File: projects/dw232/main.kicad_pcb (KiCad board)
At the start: 4 copper layers, 99 x 25 mm, 27 parts, among them P101 CONN_01X07, Q501 MMBT3904, Q502 MMBT3904, U501 LM741, U502 LM741, U503 2DW232

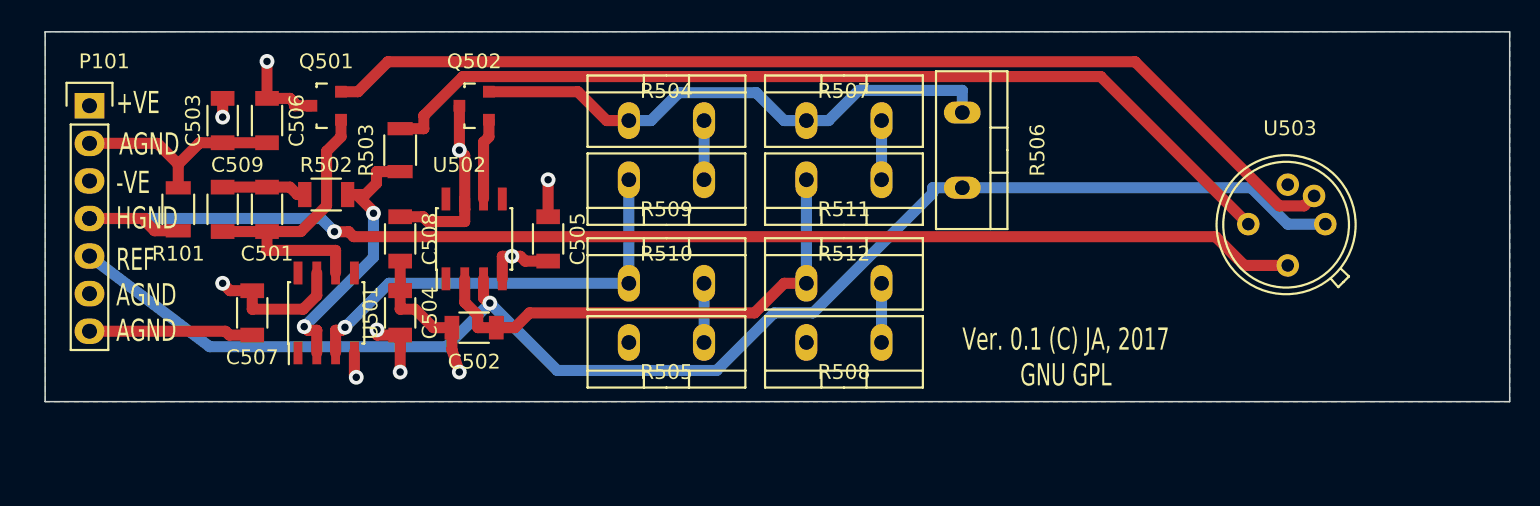
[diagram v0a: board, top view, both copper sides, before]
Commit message: adjust positions
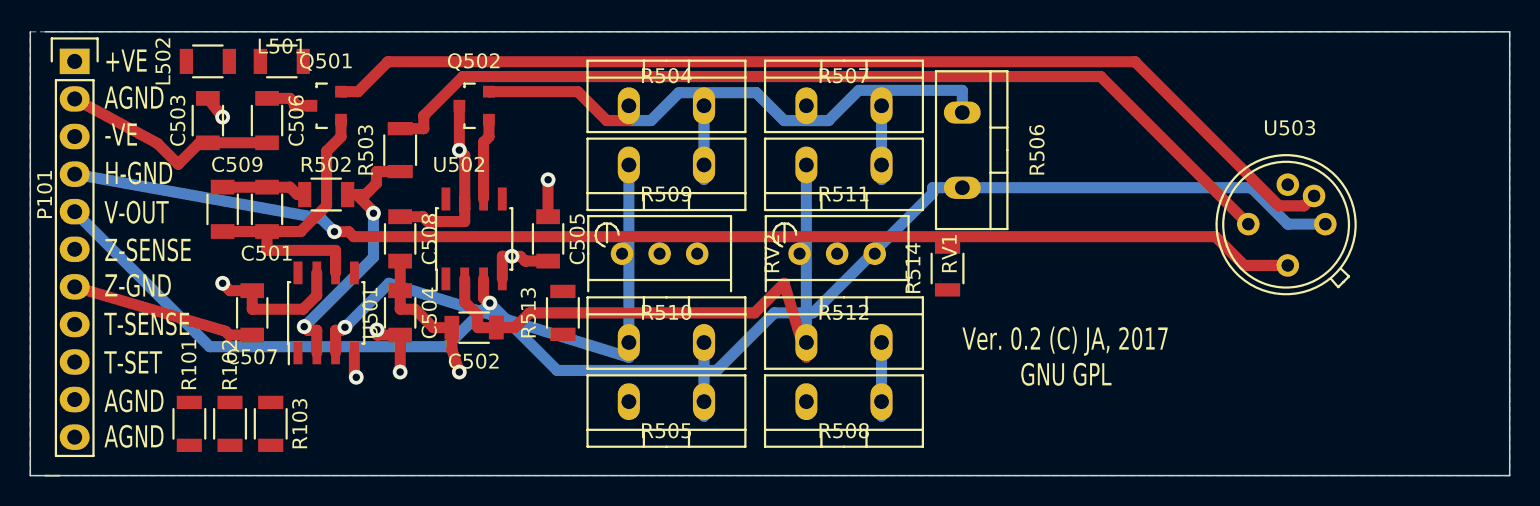
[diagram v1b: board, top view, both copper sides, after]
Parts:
- added L501: INDUCTOR, Resistors_SMD:R_1206, F.Cu at (56.0, 31.0)
- added L502: INDUCTOR, Resistors_SMD:R_1206, F.Cu at (51.0, 31.0)
- added R102: 0R, Resistors_SMD:R_1206, F.Cu at (52.5, 55.5)
- added R103: 0R, Resistors_SMD:R_1206, F.Cu at (55.2, 55.5)
- added R513: 0R, Resistors_SMD:R_1206, F.Cu at (75.0, 48.0)
- added R514: 0R, Resistors_SMD:R_1206, F.Cu at (101.0, 45.0)
- added RV1: 1k, Potentiometers:Potentiometer_Bourns_3296W_3-8Zoll_Inline_ScrewUp, F.Cu at (91.0, 44.0)
- added RV2: 1k, Potentiometers:Potentiometer_Bourns_3296W_3-8Zoll_Inline_ScrewUp, F.Cu at (79.0, 44.0)
- P101: value CONN_01X07 -> CONN_01X11; footprint Pin_Headers:Pin_Header_Straight_1x07 -> Pin_Headers:Pin_Header_Straight_1x11
- R101: value R -> 0R
- R508: value 10k -> 15k
- moved R101 14.5 mm to (49.8, 55.5), turned to 270 degrees
- moved R505 4.00 mm to (82.0, 54.0)
- moved R508 4.00 mm to (94.0, 54.0)
- moved R510 4.00 mm to (82.0, 50.0)
- moved R512 4.00 mm to (94.0, 50.0)
- moved P101 3.16 mm to (42.0, 31.0)
- moved C503 1.00 mm to (51.0, 35.0)
- moved R504 1.00 mm to (82.0, 34.0)
- moved R507 1.00 mm to (94.0, 34.0)
- moved R509 1.00 mm to (82.0, 38.0)
- moved R511 1.00 mm to (94.0, 38.0)
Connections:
- C503 pad 1: -VE -> Net-(C503-Pad1)
- C504 pad 1: -VE -> Net-(C503-Pad1)
- C505 pad 1: -VE -> Net-(C503-Pad1)
- C506 pad 1: +VE -> Net-(C506-Pad1)
- C507 pad 1: +VE -> Net-(C506-Pad1)
- C508 pad 1: +VE -> Net-(C506-Pad1)
- P101 pad 5: REF -> V-OUT
- P101 pad 6: AGND -> Z-SENSE
- P101 pad 7: AGND -> Z-SENSE-GND
- Q502 pad 2: Net-(Q502-Pad2) -> V-OUT
- R502 pad 1: Net-(R502-Pad1) -> T-SENSE
- R503 pad 1: Net-(R502-Pad1) -> T-SENSE
- R504 pad 1: Net-(Q502-Pad2) -> Z-SENSE
- R506 pad 1: Net-(Q502-Pad2) -> V-OUT
- R506 pad 2: REF -> Z-SENSE
- R507 pad 1: Net-(Q502-Pad2) -> V-OUT
- R510 pad 1: Net-(R509-Pad2) -> Net-(R510-Pad1)
- R511 pad 2: Net-(C502-Pad1) -> Net-(R511-Pad2)
- R512 pad 1: Net-(C502-Pad1) -> Net-(R512-Pad1)
- U501 pad 2: Net-(R502-Pad1) -> T-SENSE
- U501 pad 3: Net-(R509-Pad2) -> T-SET
- U502 pad 3: REF -> Z-SENSE
- U503 pad 1: REF -> Z-SENSE
- U503 pad 2: AGND -> Z-SENSE-GND
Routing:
- net REF: track 96.9 -> 0.00 mm, vias 1 -> 0
- net V-OUT: track 0.00 -> 90.1 mm, vias 0 -> 1
- net Z-SENSE: track 0.00 -> 46.3 mm
- net Net-(Q502-Pad2): track 36.7 -> 0.00 mm
- net Net-(R510-Pad1): track 0.00 -> 21.2 mm
- net T-SENSE: track 0.00 -> 18.5 mm, vias 0 -> 2
- net Net-(R502-Pad1): track 18.5 -> 0.00 mm, vias 2 -> 0
- net Net-(R509-Pad2): track 29.7 -> 12.0 mm, vias 1 -> 0
- net Net-(R511-Pad2): track 0.00 -> 12.0 mm
- net Z-SENSE-GND: track 0.00 -> 10.6 mm
- net +VE: track 28.7 -> 19.7 mm, vias 3 -> 1
- net AGND: track 38.7 -> 29.7 mm
- net Net-(C502-Pad1): track 34.1 -> 25.6 mm
- net Net-(C503-Pad1): track 0.00 -> 7.57 mm, vias 0 -> 3
- net -VE: track 12.1 -> 4.91 mm, vias 5 -> 2
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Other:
- board size 99 x 25 mm -> 100 x 30 mm
- board text added: "H-GND"
- board text added: "T-SENSE"
- board text added: "T-SET"
- board text added: "V-OUT"
- board text added: "Ver. 0.2 (C) JA, 2017 GNU GPL"
- board text added: "Z-GND"
- board text added: "Z-SENSE"
- board text removed: "HGND"
- board text removed: "REF"
- board text removed: "Ver. 0.1 (C) JA, 2017 GNU GPL"
